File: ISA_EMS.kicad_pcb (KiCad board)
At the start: 2 copper layers, 176.5 x 102.9 mm, 91 parts, among them J1 ISA BUS, J10 Parallel Port, J11 Serial 4 IDC, J12 Serial 3 IDC, J13 UART4_SEL, J14 ROM Config, J2 ADDR_IRQ, J3 UART1_SEL, J4 UART2_SEL, J5 ADDR, J6 Serial 2 IDC, J7 Serial 1 DB9, J8 UART3_SEL, J9 Parport IRQ Select, U1 74LS138, U11 74LS30, U12 74LS86, U13 74LS02, U14 74LS155, U15 74LS245, U16 74LS174, U17 74LS374, U18 74LS05, U19 74LS125, U2 74LS138, U20 74LS240, U21 74LS244, U23 16C554, U24 74LS32, U25 GD75232N, U26 GD75232N, U27 SST39SF040, U28 74HCT688, U5 GD75232N, U6 GD75232N, X1 1.8432Mhz

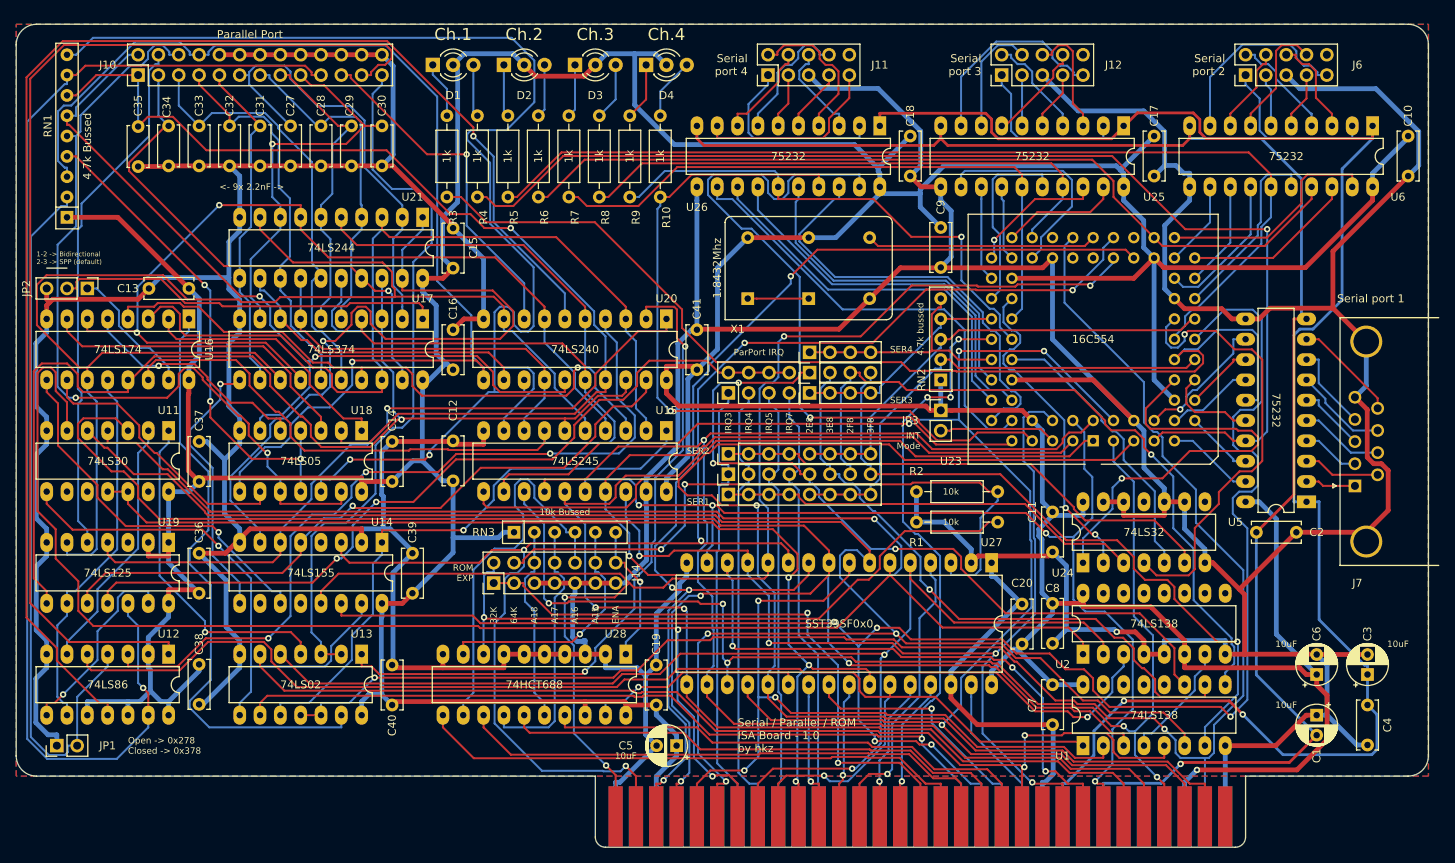
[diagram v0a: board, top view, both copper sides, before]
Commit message: Update schematic, draw board
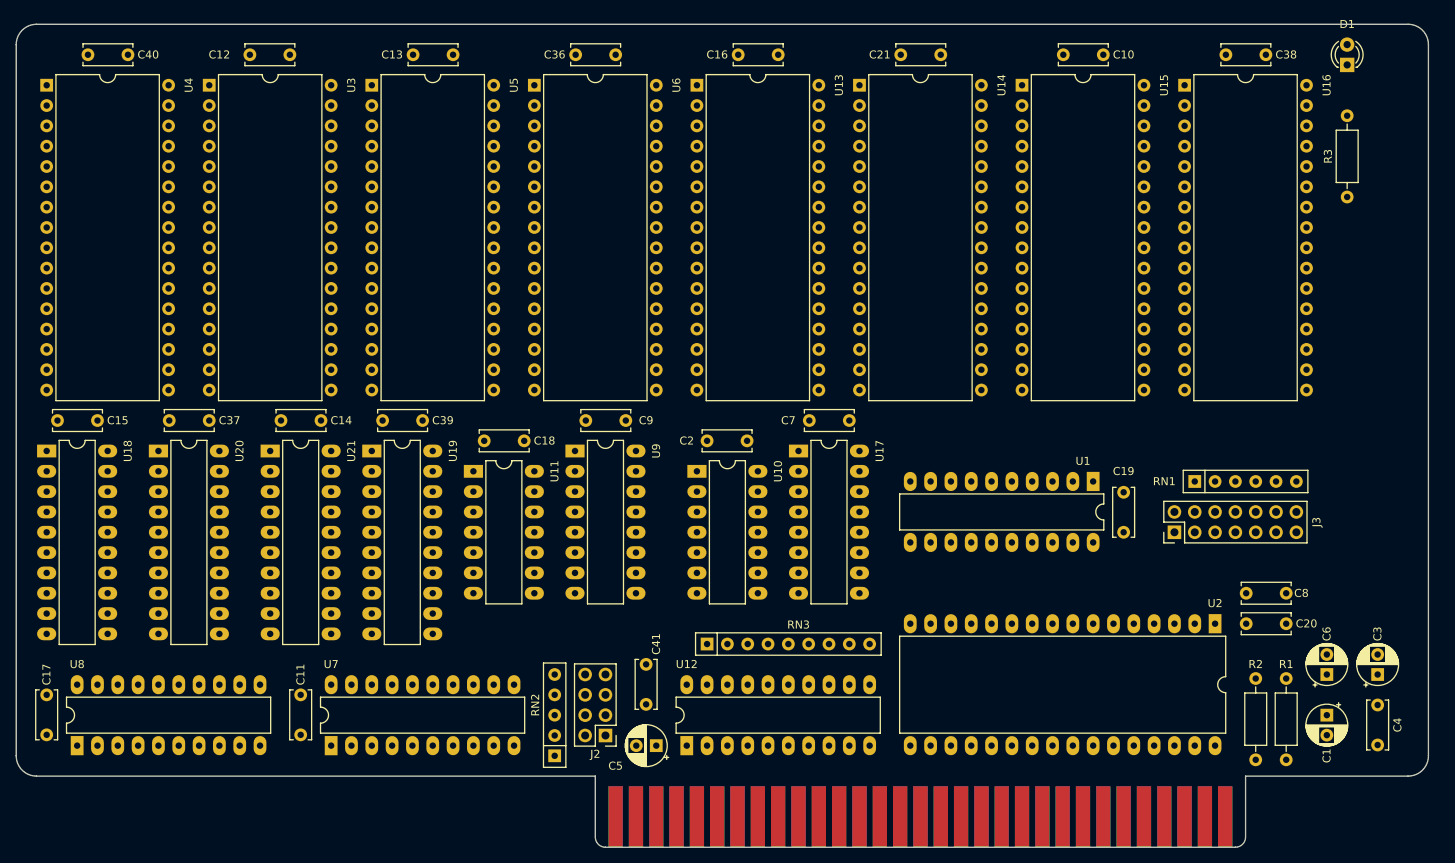
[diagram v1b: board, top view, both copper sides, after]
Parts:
- removed C27, C28, C29, C30, C31, C32, C33, C34, C35: 2.2nF, Capacitor_THT:C_Disc_D5.0mm_W2.5mm_P5.00mm
- removed D2: LED Channel B, LED_THT:LED_D3.0mm-3
- removed D3: LED Channel C, LED_THT:LED_D3.0mm-3
- removed D4: LED Channel D, LED_THT:LED_D3.0mm-3
- removed J10: Parallel Port, Connector_PinHeader_2.54mm:PinHeader_2x13_P2.54mm_Vertical
- removed J11: Serial 4 IDC, Connector_PinHeader_2.54mm:PinHeader_2x05_P2.54mm_Vertical
- removed J12: Serial 3 IDC, Connector_PinHeader_2.54mm:PinHeader_2x05_P2.54mm_Vertical
- removed J13: UART4_SEL, Connector_PinHeader_2.54mm:PinHeader_1x04_P2.54mm_Vertical
- removed the J3 at (227.4, 159.1)
- removed J4: UART2_SEL, Connector_PinHeader_2.54mm:PinHeader_1x08_P2.54mm_Vertical
- removed J5: ADDR, Connector_PinHeader_2.54mm:PinHeader_1x04_P2.54mm_Vertical
- removed J6: Serial 2 IDC, Connector_PinHeader_2.54mm:PinHeader_2x05_P2.54mm_Vertical
- removed J7: Serial 1 DB9, Connector_Dsub:DSUB-9_Male_Horizontal_P2.77x2.84mm_EdgePinOffset7.70mm_Housed_MountingHolesOffset9.12mm
- removed J8: UART3_SEL, Connector_PinHeader_2.54mm:PinHeader_1x04_P2.54mm_Vertical
- removed J9: Parport IRQ Select, Connector_PinHeader_2.54mm:PinHeader_2x04_P2.54mm_Vertical
- removed JP1: Address selection, Connector_PinHeader_2.54mm:PinHeader_1x02_P2.54mm_Vertical
- removed JP2: Parport type, Connector_PinHeader_2.54mm:PinHeader_1x03_P2.54mm_Vertical
- removed JP3: Interrupt Mode, Connector_PinHeader_2.54mm:PinHeader_1x02_P2.54mm_Vertical
- removed R10, R4, R5, R6, R7, R8, R9: 1k, Resistor_THT:R_Axial_DIN0207_L6.3mm_D2.5mm_P10.16mm_Horizontal
- removed the RN1 at (144.8, 124.5)
- removed the U1 at (271.8, 190.5)
- removed the U2 at (271.8, 179.1)
- removed U23: 16C554, Package_LCC:PLCC-68_THT-Socket
- removed U24: 74LS32, Package_DIP:DIP-14_W7.62mm_LongPads
- removed U25, U26: GD75232N, Package_DIP:DIP-20_W7.62mm_LongPads
- removed X1: 1.8432Mhz, ISA_DualUART:Oscillator_DIP-14-8
- added C21: 100nF, Capacitor_THT:C_Disc_D6.0mm_W2.5mm_P5.00mm, F.Cu at (254.0, 104.1)
- added RN3: 10k, Resistor_THT:R_Array_SIP9, F.Cu at (224.8, 177.8)
- added U10: 74HCT32, Package_DIP:DIP-14_W7.62mm_LongPads, F.Cu at (223.5, 156.2)
- added U3: AS6C4008-55PCN, Package_DIP:DIP-32_W15.24mm, F.Cu at (162.6, 108.0)
- added U4: AS6C4008-55PCN, Package_DIP:DIP-32_W15.24mm, F.Cu at (142.2, 108.0)
- added U7: 74HCT688, Package_DIP:DIP-20_W7.62mm_LongPads, F.Cu at (177.8, 190.5)
- added U8: 74HCT688, Package_DIP:DIP-20_W7.62mm_LongPads, F.Cu at (146.1, 190.5)
- added U9: 74HCT139, Package_DIP:DIP-16_W7.62mm_LongPads, F.Cu at (208.3, 153.7)
- D1: value LED Channel A -> EMS in use; footprint LED_THT:LED_D3.0mm-3 -> LED_THT:LED_D3.0mm_Clear
- J2: value ADDR_IRQ -> EMS Address; footprint Connector_PinHeader_2.54mm:PinHeader_1x08_P2.54mm_Vertical -> Connector_PinHeader_2.54mm:PinHeader_2x04_P2.54mm_Vertical
- RN2: value 4.7k -> 10k
- U11: value 74LS30 -> 74HCT04
- U12: value 74LS86 -> 74ACT245; footprint Package_DIP:DIP-14_W7.62mm_LongPads -> Package_DIP:DIP-20_W7.62mm_LongPads
- U13: value 74LS02 -> AS6C4008-55PCN; footprint Package_DIP:DIP-14_W7.62mm_LongPads -> Package_DIP:DIP-32_W15.24mm
- U14: value 74LS155 -> AS6C4008-55PCN; footprint Package_DIP:DIP-16_W7.62mm_LongPads -> Package_DIP:DIP-32_W15.24mm
- U15: value 74LS245 -> AS6C4008-55PCN; footprint Package_DIP:DIP-20_W7.62mm_LongPads -> Package_DIP:DIP-32_W15.24mm
- U16: value 74LS174 -> AS6C4008-55PCN; footprint Package_DIP:DIP-16_W7.62mm_LongPads -> Package_DIP:DIP-32_W15.24mm
- U17: value 74LS374 -> 74HCT138; footprint Package_DIP:DIP-20_W7.62mm_LongPads -> Package_DIP:DIP-16_W7.62mm_LongPads
- U18: value 74LS05 -> 74LS573; footprint Package_DIP:DIP-14_W7.62mm_LongPads -> Package_DIP:DIP-20_W7.62mm_LongPads
- U19: value 74LS125 -> 74LS573; footprint Package_DIP:DIP-14_W7.62mm_LongPads -> Package_DIP:DIP-20_W7.62mm_LongPads
- U20: value 74LS240 -> 74LS573
- U21: value 74LS244 -> 74LS573
- U5, U6: value GD75232N -> AS6C4008-55PCN; footprint Package_DIP:DIP-20_W7.62mm_LongPads -> Package_DIP:DIP-32_W15.24mm
- moved C17 155.1 mm to (142.2, 184.2)
- moved C38 153.6 mm to (294.6, 104.1), turned to 180 degrees
- moved U5 127.9 mm to (182.9, 108.0), turned to 0 degrees
- moved U16 127.8 mm to (284.5, 108.0), turned to 0 degrees
- moved D1 114.3 mm to (304.8, 105.4), turned to 90 degrees
- moved R3 113.0 mm to (304.8, 121.9), turned to 90 degrees
- moved U6 104.9 mm to (203.2, 108.0), turned to 0 degrees
- moved C11 96.7 mm to (174.0, 184.2)
- moved C40 87.7 mm to (152.4, 104.1), turned to 180 degrees
- moved RN1 85.3 mm to (285.8, 157.5)
- moved J3 85.3 mm to (283.2, 163.8)
- moved C36 85.1 mm to (213.4, 104.1), turned to 180 degrees
- moved U14 82.6 mm to (243.8, 108.0), turned to 0 degrees
- moved U13 82.5 mm to (223.5, 108.0), turned to 0 degrees
- moved C2 74.5 mm to (224.8, 152.4), turned to 0 degrees
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- renumbered J14 to J3, RN3 to RN1, U28 to U1, U27 to U2
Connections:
- J1 pad 14: /~IOR -> (no net)
- J1 pad 2: /RESETDRV -> (no net)
- J1 pad 21: /IRQ7 -> (no net)
- J1 pad 23: /IRQ5 -> (no net)
- J1 pad 24: /IRQ4 -> (no net)
- J1 pad 25: /IRQ3 -> (no net)
- J2 pad 1: /IRQ3 -> GND
- J2 pad 2: /IRQ4 -> /JP1
- J2 pad 3: /IRQ5 -> GND
- J2 pad 4: /IRQ7 -> /JP2
- J2 pad 5: /0x2E8 -> GND
- J2 pad 6: /0x3E8 -> /JP3
- J2 pad 7: /0x2F8 -> GND
- J2 pad 8: /0x3F8 -> /JP4
- R3 pad 1: Net-(D1-Pad1) -> /~RAM-SELECT
- R3 pad 2: /TX_A -> Net-(D1-Pad1)
- RN2 pad 2: /~UART1_CS -> /JP1
- RN2 pad 3: /~UART2_CS -> /JP2
- RN2 pad 4: /~UART3_CS -> /JP3
- RN2 pad 5: /~UART4_CS -> /JP4
- U11 pad 11: /A9 -> GND
- U11 pad 12: /A9 -> (no net)
- U11 pad 13: (no net) -> GND
- U11 pad 2: Net-(U11-Pad2) -> /REG0-LOAD
- U11 pad 3: /A3 -> Net-(U11-Pad3)
- U11 pad 4: /A4 -> /REG1-LOAD
- U11 pad 5: /A5 -> Net-(U11-Pad5)
- U11 pad 6: /A6 -> /REG2-LOAD
- U11 pad 8: Net-(U11-Pad8) -> /REG3-LOAD
- U11 pad 9: (no net) -> Net-(U11-Pad9)
- U12 pad 1: /PARPORT_PE -> /~MEMR
- U12 pad 10: VCC -> GND
- U12 pad 11: /PARPORT_IRQ -> /DB7
- U12 pad 12: VCC -> /DB6
- U12 pad 13: /RN_7 -> /DB5
- U12 pad 14: VCC -> /DB4
- U12 pad 2: VCC -> /D0
- U12 pad 3: Net-(U12-Pad3) -> /D1
- U12 pad 4: /RN_1 -> /D2
- U12 pad 5: /A8 -> /D3
- U12 pad 6: Net-(U11-Pad2) -> /D4
- U12 pad 7: GND -> /D5
- U12 pad 8: /~PARPORT_IRQEN -> /D6
- U12 pad 9: /PARPORT_IRQEN -> /D7
- U13 pad 1: Net-(U13-Pad1) -> /RAM-A18
- U13 pad 10: /PARPORT_R -> /A2
- U13 pad 11: /RESETDRV -> /A1
- U13 pad 12: /RESETDRV -> /A0
- U13 pad 13: /~PARPORT_RESET -> /DB0
- U13 pad 14: VCC -> /DB1
- U13 pad 2: /PARPORT_SLCT -> /RAM-A16
- U13 pad 3: /PARPORT_SLCT -> /RAM-A14
- U13 pad 4: Net-(U11-Pad1) -> /A12
- U13 pad 6: /AEN -> /A6
- U13 pad 7: GND -> /A5
- U13 pad 8: Net-(U11-Pad8) -> /A4
- U13 pad 9: /~IOR -> /A3
- U14 pad 1: /PARPORT_R -> /RAM-A18
- U14 pad 10: (no net) -> /A2
- U14 pad 11: /PARPORT_WPC -> /A1
- U14 pad 12: (no net) -> /A0
- U14 pad 13: /A0 -> /DB0
- U14 pad 14: /~IOW -> /DB1
- U14 pad 15: Net-(U11-Pad8) -> /DB2
- U14 pad 16: VCC -> GND
- U14 pad 2: GND -> /RAM-A16
- U14 pad 3: /A1 -> /RAM-A14
- U14 pad 4: (no net) -> /A12
- U14 pad 5: /PARPORT_RPC -> /A7
- U14 pad 6: /PARPORT_RPB -> /A6
- U14 pad 7: /PARPORT_RPA -> /A5
- U14 pad 8: GND -> /A4
- U14 pad 9: /PARPORT_WPA -> /A3
- U15 pad 1: /PARPORT_R -> /RAM-A18
- U15 pad 10: GND -> /A2
- U15 pad 11: /D7 -> /A1
- U15 pad 12: /D6 -> /A0
- U15 pad 13: /D5 -> /DB0
- U15 pad 14: /D4 -> /DB1
- U15 pad 15: /D3 -> /DB2
- U15 pad 16: /D2 -> GND
- U15 pad 17: /D1 -> /DB3
- U15 pad 18: /D0 -> /DB4
- U15 pad 19: GND -> /DB5
- U15 pad 2: /PARPORT_BD0 -> /RAM-A16
- U15 pad 20: VCC -> /DB6
- U15 pad 3: /PARPORT_BD1 -> /RAM-A14
- U15 pad 4: /PARPORT_BD2 -> /A12
- U15 pad 5: /PARPORT_BD3 -> /A7
- U15 pad 6: /PARPORT_BD4 -> /A6
- U15 pad 7: /PARPORT_BD5 -> /A5
- U15 pad 8: /PARPORT_BD6 -> /A4
- U15 pad 9: /PARPORT_BD7 -> /A3
- U16 pad 1: /~PARPORT_RESET -> /RAM-A18
- U16 pad 10: Net-(U16-Pad10) -> /A2
- U16 pad 11: /PARPORT_BD3 -> /A1
- U16 pad 12: /PARPORT_IRQEN -> /A0
- U16 pad 13: /PARPORT_BD4 -> /DB0
- U16 pad 14: /PARPORT_BD5 -> /DB1
- U16 pad 15: /PARPORT_DIR -> /DB2
- U16 pad 16: VCC -> GND
- U16 pad 2: Net-(U16-Pad2) -> /RAM-A16
- U16 pad 3: /PARPORT_BD0 -> /RAM-A14
- U16 pad 4: /PARPORT_BD1 -> /A12
- U16 pad 5: Net-(U16-Pad5) -> /A7
- U16 pad 6: /PARPORT_BD2 -> /A6
- U16 pad 7: Net-(U16-Pad7) -> /A5
- U16 pad 8: GND -> /A4
- U16 pad 9: /PARPORT_WPC -> /A3
- U17 pad 1: Net-(JP2-Pad2) -> /RAM-A19
- U17 pad 10: GND -> /~RAM-CS5
- U17 pad 11: /PARPORT_WPA -> /~RAM-CS4
- U17 pad 12: /PARPORT_DATA3 -> /~RAM-CS3
- U17 pad 13: /PARPORT_BD3 -> /~RAM-CS2
- U17 pad 14: /PARPORT_BD2 -> /~RAM-CS1
- U17 pad 15: /PARPORT_DATA2 -> /~RAM-CS0
- U17 pad 16: /PARPORT_DATA1 -> VCC
- U17 pad 2: /PARPORT_DATA4 -> /RAM-A20
- U17 pad 3: /PARPORT_BD4 -> /RAM-A21
- U17 pad 4: /PARPORT_BD5 -> GND
- U17 pad 5: /PARPORT_DATA5 -> /~RAM-SELECT
- U17 pad 6: /PARPORT_DATA6 -> VCC
- U17 pad 7: /PARPORT_BD6 -> /~RAM-CS7
- U17 pad 8: /PARPORT_BD7 -> GND
- U17 pad 9: /PARPORT_DATA7 -> /~RAM-CS6
- U18 pad 1: Net-(U16-Pad2) -> /~REG0-OE
- U18 pad 10: /RN_4 -> GND
- U18 pad 11: /RN_3 -> /REG0-LOAD
- U18 pad 12: /RN_8 -> /RAM-A21
- U18 pad 13: /RN_4 -> /RAM-A20
- U18 pad 14: VCC -> /RAM-A19
- U18 pad 2: /RN_6 -> /D0
- U18 pad 3: Net-(U16-Pad7) -> /D1
- U18 pad 4: /RN_3 -> /D2
- U18 pad 5: Net-(U16-Pad5) -> /D3
- U18 pad 6: /RN_5 -> /D4
- U18 pad 7: GND -> /D5
- U18 pad 8: /RN_2 -> /D6
- U18 pad 9: Net-(U16-Pad10) -> /D7
- U19 pad 1: VCC -> /~REG1-OE
- U19 pad 10: /PARPORT_RPC -> GND
- U19 pad 11: Net-(J9-Pad2) -> /REG1-LOAD
- U19 pad 12: /RN_7 -> /RAM-A21
- U19 pad 13: /~PARPORT_IRQEN -> /RAM-A20
- U19 pad 14: VCC -> /RAM-A19
- U19 pad 2: VCC -> /D0
- U19 pad 3: (no net) -> /D1
- U19 pad 4: /PARPORT_RPB -> /D2
- U19 pad 5: /~PARPORT_ERROR -> /D3
- U19 pad 6: /PARPORT_BD3 -> /D4
- U19 pad 7: GND -> /D5
- U19 pad 8: /PARPORT_BD4 -> /D6
- U19 pad 9: /PARPORT_IRQEN -> /D7
- U20 pad 1: /PARPORT_RPB -> /~REG2-OE
- U20 pad 11: /RN_2 -> /REG2-LOAD
- U20 pad 12: /PARPORT_BD7 -> /RAM-A21
- U20 pad 13: /RN_8 -> /RAM-A20
- U20 pad 14: /PARPORT_BD6 -> /RAM-A19
- U20 pad 15: /RN_5 -> /RAM-A18
- U20 pad 16: /PARPORT_BD5 -> /RAM-A17
- U20 pad 17: /RN_6 -> /RAM-A16
- U20 pad 18: /PARPORT_BD4 -> /RAM-A15
- U20 pad 19: /PARPORT_RPC -> /RAM-A14
- U20 pad 2: Net-(U13-Pad1) -> /D0
- U20 pad 3: /PARPORT_BD0 -> /D1
- U20 pad 4: Net-(U12-Pad3) -> /D2
- U20 pad 5: /PARPORT_BD1 -> /D3
- U20 pad 6: /PARPORT_IRQ -> /D4
- U20 pad 7: /PARPORT_BD2 -> /D5
- U20 pad 8: /PARPORT_BUSY -> /D6
- U20 pad 9: /PARPORT_BD3 -> /D7
- U21 pad 1: /PARPORT_RPA -> /~REG3-OE
- U21 pad 11: /PARPORT_DATA3 -> /REG3-LOAD
- U21 pad 12: /PARPORT_BD7 -> /RAM-A21
- U21 pad 13: /PARPORT_DATA2 -> /RAM-A20
- U21 pad 14: /PARPORT_BD6 -> /RAM-A19
- U21 pad 15: /PARPORT_DATA1 -> /RAM-A18
- U21 pad 16: /PARPORT_BD5 -> /RAM-A17
- U21 pad 17: /PARPORT_DATA0 -> /RAM-A16
- U21 pad 18: /PARPORT_BD4 -> /RAM-A15
- U21 pad 19: /PARPORT_RPA -> /RAM-A14
- U21 pad 2: /PARPORT_DATA4 -> /D0
- U21 pad 3: /PARPORT_BD0 -> /D1
- U21 pad 4: /PARPORT_DATA5 -> /D2
- U21 pad 5: /PARPORT_BD1 -> /D3
- U21 pad 6: /PARPORT_DATA6 -> /D4
- U21 pad 7: /PARPORT_BD2 -> /D5
- U21 pad 8: /PARPORT_DATA7 -> /D6
- U21 pad 9: /PARPORT_BD3 -> /D7
- U5 pad 1: +12V -> /RAM-A18
- U5 pad 10: -12V -> /A2
- U5 pad 11: GND -> /A1
- U5 pad 12: /~RI_A -> /A0
- U5 pad 13: /~DTR_A -> /DB0
- U5 pad 14: /~CTS_A -> /DB1
- U5 pad 15: /TX_A -> /DB2
- U5 pad 16: /~RTS_A -> GND
- U5 pad 17: /RX_A -> /DB3
- U5 pad 18: /~DSR_A -> /DB4
- U5 pad 19: /~DCD_A -> /DB5
- U5 pad 2: /RS232_1_DCD -> /RAM-A16
- U5 pad 20: VCC -> /DB6
- U5 pad 3: /RS232_1_DSR -> /RAM-A14
- U5 pad 4: /RS232_1_RX -> /A12
- U5 pad 5: /RS232_1_RTS -> /A7
- U5 pad 6: /RS232_1_TX -> /A6
- U5 pad 7: /RS232_1_CTS -> /A5
- U5 pad 8: /RS232_1_DTR -> /A4
- U5 pad 9: /RS232_1_RI -> /A3
- U6 pad 1: +12V -> /RAM-A18
- U6 pad 10: -12V -> /A2
- U6 pad 11: GND -> /A1
- U6 pad 12: /~RI_B -> /A0
- U6 pad 13: /~DTR_B -> /DB0
- U6 pad 14: /~CTS_B -> /DB1
- U6 pad 15: /TX_B -> /DB2
- U6 pad 16: /~RTS_B -> GND
- U6 pad 17: /RX_B -> /DB3
- U6 pad 18: /~DSR_B -> /DB4
- U6 pad 19: /~DCD_B -> /DB5
- U6 pad 2: /RS232_2_DCD -> /RAM-A16
- U6 pad 20: VCC -> /DB6
- U6 pad 3: /RS232_2_DSR -> /RAM-A14
- U6 pad 4: /RS232_2_RX -> /A12
- U6 pad 5: /RS232_2_RTS -> /A7
- U6 pad 6: /RS232_2_TX -> /A6
- U6 pad 7: /RS232_2_CTS -> /A5
- U6 pad 8: /RS232_2_DTR -> /A4
- U6 pad 9: /RS232_2_RI -> /A3
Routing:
- net GND: track 995.6 -> 0.00 mm, vias 1 -> 0
- net VCC: track 784.3 -> 0.00 mm, vias 1 -> 0
- net /~IOW: track 221.8 -> 0.00 mm, vias 5 -> 0
- net /A5: track 215.0 -> 0.00 mm, vias 3 -> 0
- net /A3: track 214.5 -> 0.00 mm, vias 3 -> 0
- net +12V: track 212.6 -> 0.00 mm, vias 2 -> 0
- net /A4: track 211.9 -> 0.00 mm, vias 4 -> 0
- net /RESETDRV: track 209.8 -> 0.00 mm, vias 2 -> 0
- net /A6: track 206.4 -> 0.00 mm, vias 2 -> 0
- net /D6: track 204.3 -> 0.00 mm, vias 4 -> 0
- net -12V: track 195.6 -> 0.00 mm, vias 1 -> 0
- net /A1: track 190.6 -> 0.00 mm, vias 5 -> 0
- net /D7: track 189.2 -> 0.00 mm, vias 1 -> 0
- net /A0: track 176.4 -> 0.00 mm, vias 4 -> 0
- net /PARPORT_IRQ: track 175.4 -> 0.00 mm, vias 1 -> 0
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- removed copper zone on B.Cu, net GND
- removed copper zone on F.Cu, net GND
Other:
- board text removed: "1-2 -> Bidirectional 2-3 -> SPP (default)"
- board text removed: "1.8432Mhz"
- board text removed: "10k"
- board text removed: "10k Bussed"
- board text removed: "10uF"
- board text removed: "16C554"
- board text removed: "1k"
- board text removed: "2E8"
- board text removed: "2F8"
- board text removed: "32K"
- board text removed: "3E8"
- board text removed: "3F8"
- board text removed: "4.7k Bussed"
- board text removed: "4.7k bussed"
- board text removed: "64K"
- board text removed: "74HCT688"
- board text removed: "74LS02"
- board text removed: "74LS05"
- board text removed: "74LS125"
- board text removed: "74LS138"
- board text removed: "74LS155"
- board text removed: "74LS174"
- board text removed: "74LS240"
- board text removed: "74LS244"
- board text removed: "74LS245"
- board text removed: "74LS30"
- board text removed: "74LS32"
- board text removed: "74LS374"
- board text removed: "74LS86"
- board text removed: "75232"
- board text removed: "<- 9x 2.2nF ->"
- board text removed: "A15"
- board text removed: "A16"
- board text removed: "A17"
- board text removed: "A18"
- board text removed: "Ch.1"
- board text removed: "Ch.2"
- board text removed: "Ch.3"
- board text removed: "Ch.4"
- board text removed: "ENA"
- board text removed: "INT Mode"
- board text removed: "IRQ3"
- board text removed: "IRQ4"
- board text removed: "IRQ5"
- board text removed: "IRQ7"
- board text removed: "Open -> 0x278 Closed -> 0x378"
- board text removed: "ParPort IRQ"
- board text removed: "Parallel Port"
- board text removed: "ROM EXP"
- board text removed: "SER1"
- board text removed: "SER2"
- board text removed: "SER3"
- board text removed: "SER4"
- board text removed: "SST39SF0x0"
- board text removed: "Serial / Parallel / ROM ISA Board - 1.0 by hkz"
- board text removed: "Serial port 1"
- board text removed: "Serial port 2"
- board text removed: "Serial port 3"
- board text removed: "Serial port 4"
